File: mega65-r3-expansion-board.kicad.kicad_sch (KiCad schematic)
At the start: 0 parts

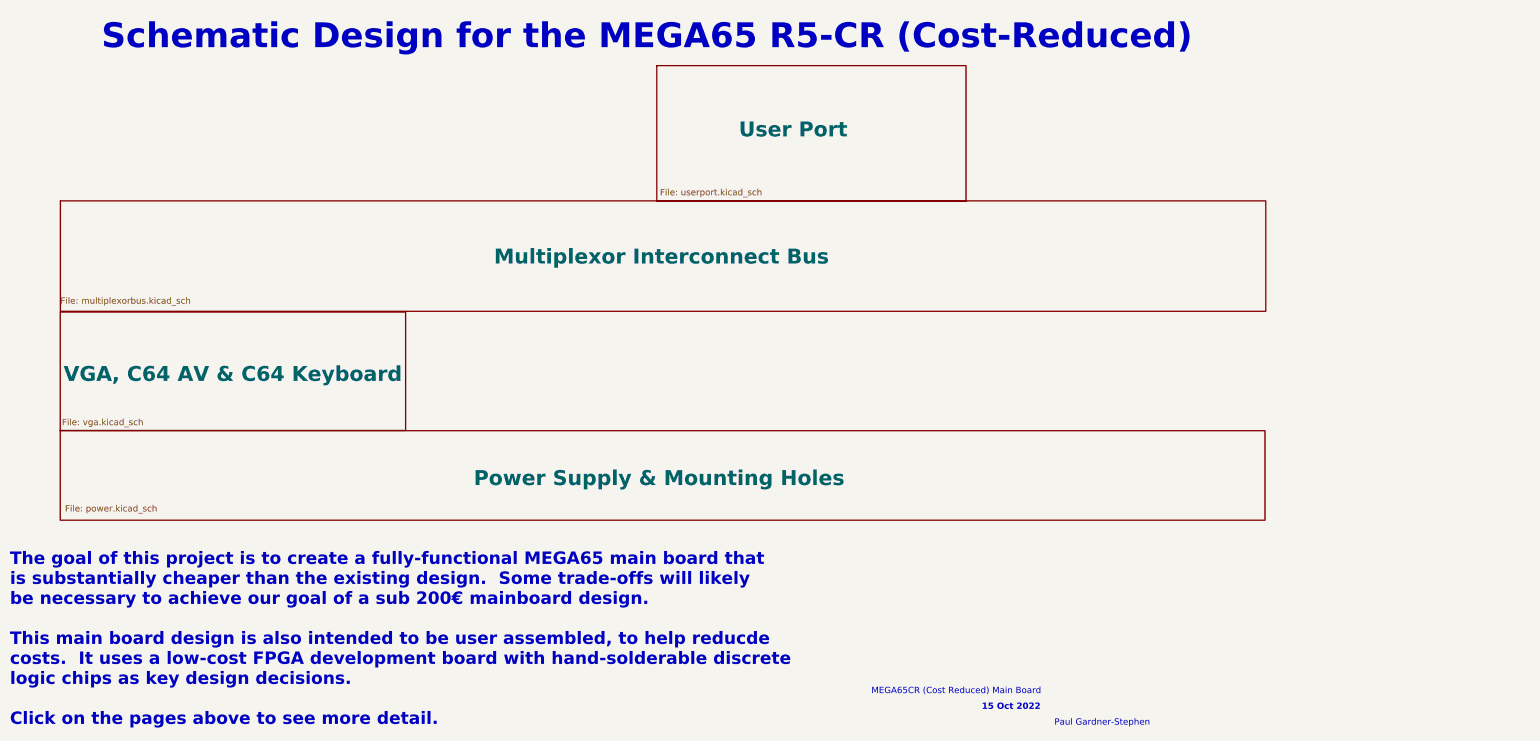
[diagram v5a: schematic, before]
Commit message: update master sheet for schematics
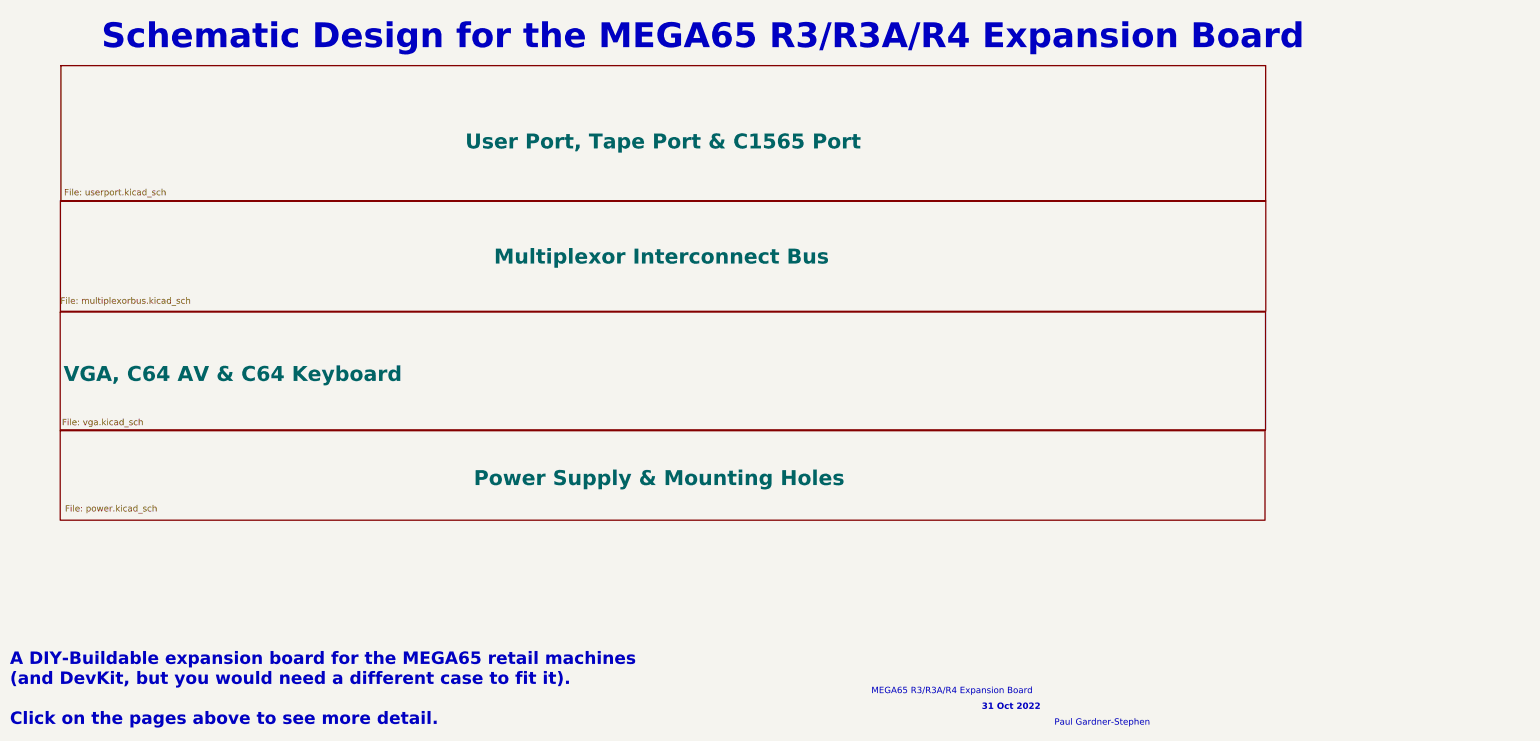
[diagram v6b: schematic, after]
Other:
- sheet User Port renamed User Port, Tape Port & C1565 Port
- note added: "31 Oct 2022"
- note added: "A DIY-Buildable expansion board for the MEGA65 retail machines (and DevKit, but you would need a different case to fit it). Click on the pages above to see more detail."
- note added: "MEGA65 R3/R3A/R4 Expansion Board"
- note added: "Schematic Design for the MEGA65 R3/R3A/R4 Expansion Board"
- note removed: "15 Oct 2022"
- note removed: "MEGA65CR (Cost Reduced) Main Board"
- note removed: "Schematic Design for the MEGA65 R5-CR (Cost-Reduced)"
- note removed: "The goal of this project is to create a fully-functional MEGA65 main board that is substantially cheaper than the existing design. Some trade-offs will likely be necessary to achieve our goal of a sub 200€ mainboard design. This main board design is also intended to be user assembled, to help reducde costs. It uses a low-cost FPGA development board with hand-solderable discrete logic chips as key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"
